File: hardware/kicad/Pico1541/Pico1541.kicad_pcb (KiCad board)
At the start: 2 copper layers, 100 x 76.2 mm, 64 parts, among them J1 SWD, J2 Serial, J3 Display/Keys, J4 Micro SD Card, J5 5V_EXT, J6 USB_A, J7 OLED/Key_Hat, J8 OLED, J9 DIN-6, Q1 MMBT3904, SW1 Reset, SW2 Button1, SW3 Button3, SW4 Button2, SW5 Button4, U1 74LS05, U2 SRV05-4

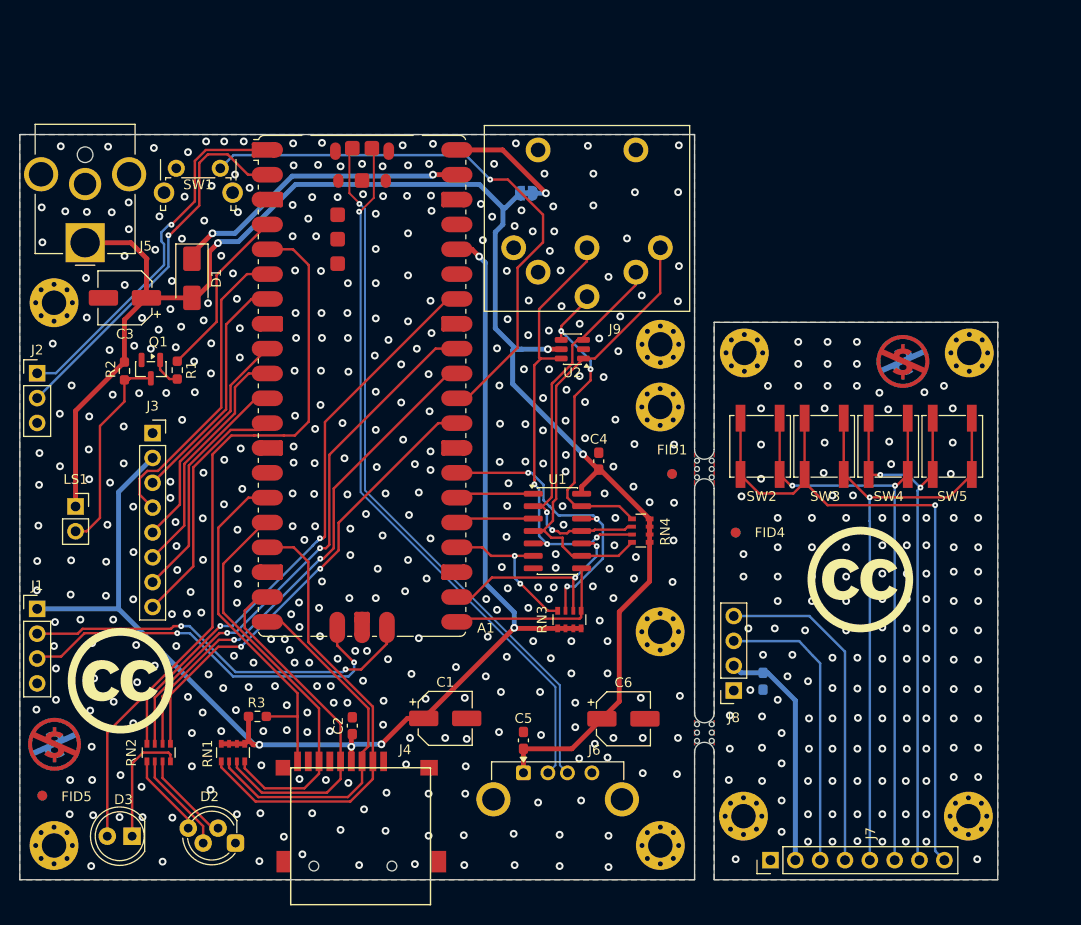
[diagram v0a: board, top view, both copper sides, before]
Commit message: Added Gerber files for final design for JLCPCB.
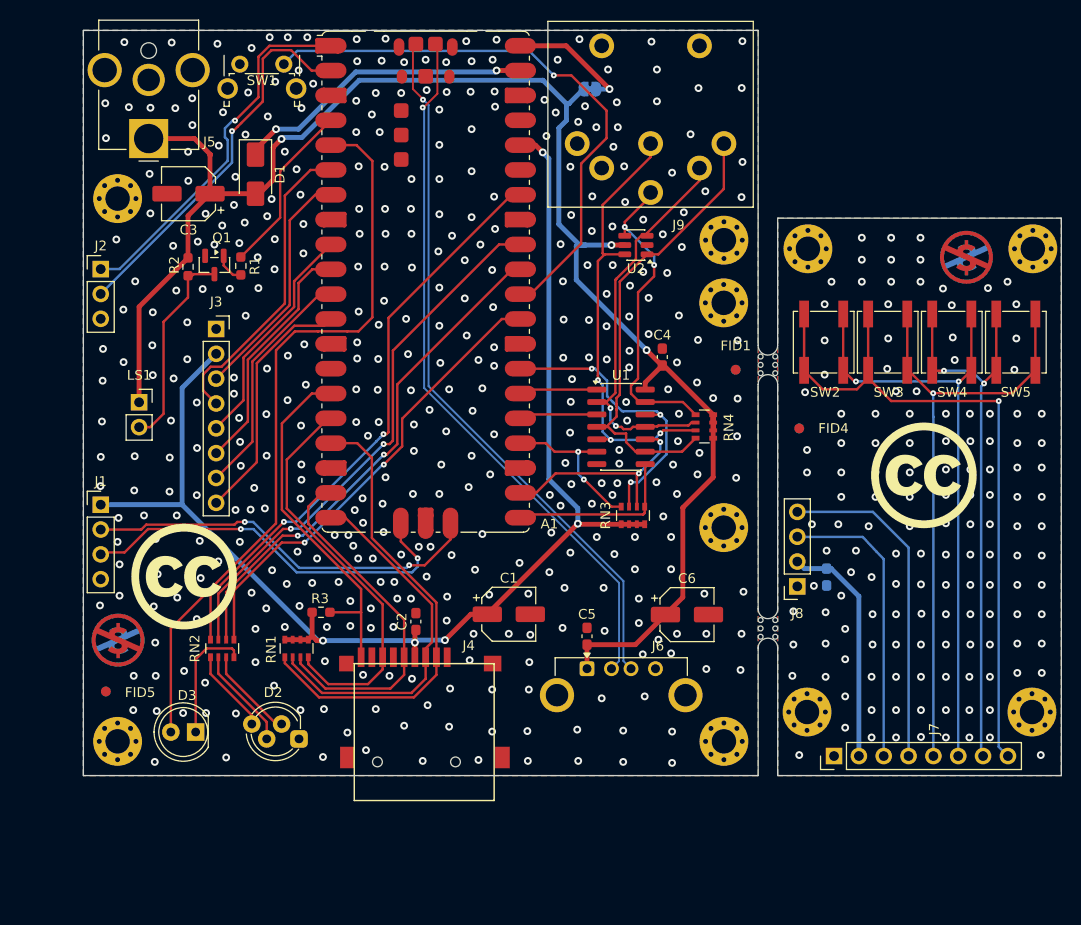
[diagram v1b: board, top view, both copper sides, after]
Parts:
- moved A1 12.5 mm to (134.0, 78.8)
- moved C1 12.5 mm to (142.5, 112.8)
- moved C2 12.5 mm to (133.0, 113.6)
- moved C3 12.5 mm to (109.8, 69.8)
- moved C4 12.5 mm to (158.2, 86.5)
- moved C5 12.5 mm to (150.5, 115.1)
- moved C6 12.5 mm to (160.7, 112.9)
- moved C7 12.5 mm to (175.0, 109.0)
- moved D1 12.5 mm to (116.6, 67.8)
- moved D2 12.5 mm to (121.0, 125.6)
- moved D3 12.5 mm to (110.5, 124.9)
- moved FID1 12.5 mm to (165.7, 87.8)
- moved FID2 12.5 mm to (165.7, 87.8)
- moved FID3 12.5 mm to (172.2, 93.8)
- moved FID4 12.5 mm to (172.2, 93.8)
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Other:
- outline, holes or cut-outs redrawn
